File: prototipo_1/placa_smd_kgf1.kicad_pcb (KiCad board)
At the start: 2 copper layers, 30 x 35 mm, 10 parts, among them J1 Conn_01x01_Female, J2 Conn_01x03_Female, J3 Conn_01x01_Female

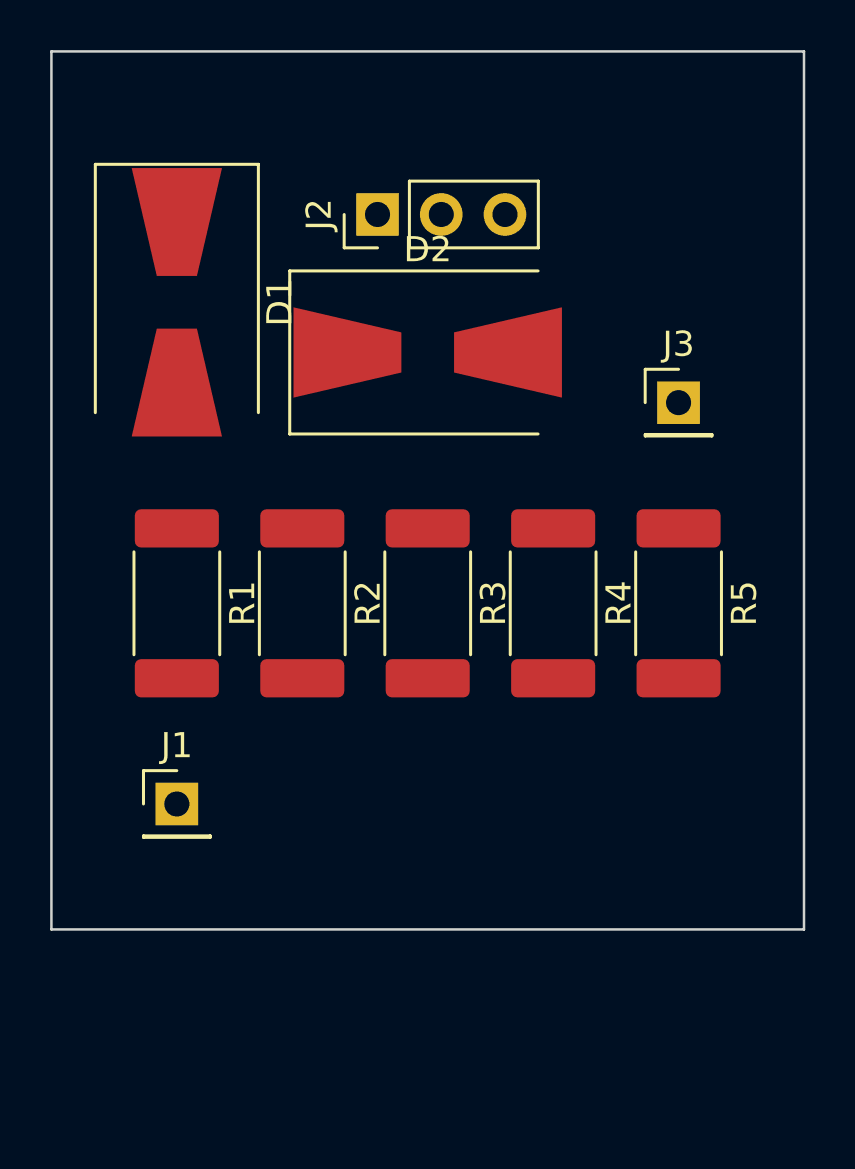
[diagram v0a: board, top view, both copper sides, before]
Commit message: Actualizacion de prototipo
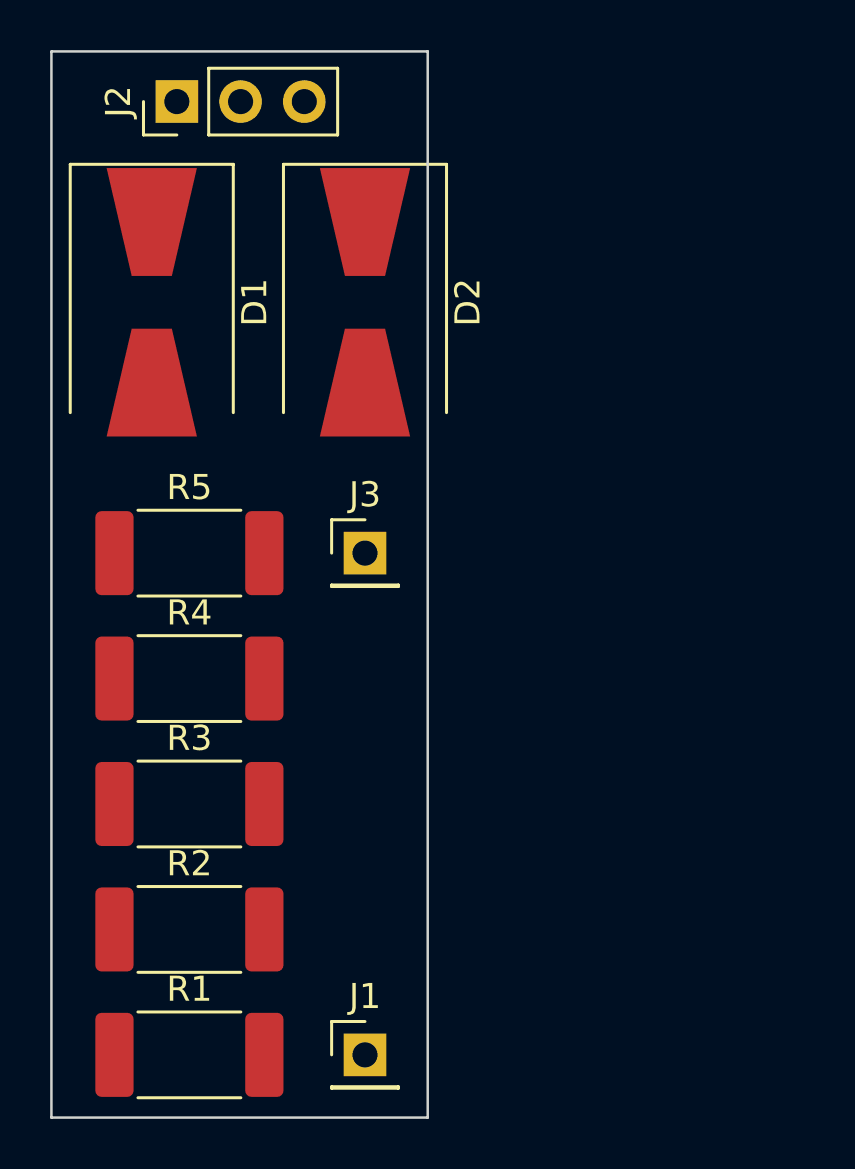
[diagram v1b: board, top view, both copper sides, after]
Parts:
- moved R5 19.6 mm to (125.5, 90.0), turned to 0 degrees
- moved R1 18.0 mm to (125.5, 110.0), turned to 0 degrees
- moved R4 14.8 mm to (125.5, 95.0), turned to 0 degrees
- moved J3 13.9 mm to (132.5, 90.0)
- moved R2 13.8 mm to (125.5, 105.0), turned to 0 degrees
- moved J1 12.5 mm to (132.5, 110.0)
- moved R3 12.4 mm to (125.5, 100.0), turned to 0 degrees
- moved J2 9.18 mm to (125.0, 72.0)
- moved D2 3.20 mm to (132.5, 80.0), turned to 270 degrees
- moved D1 1.00 mm to (124.0, 80.0)
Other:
- board size 30 x 35 mm -> 15 x 42.5 mm
